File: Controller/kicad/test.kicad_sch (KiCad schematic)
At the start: 21 parts, among them J13 TEST POINTS

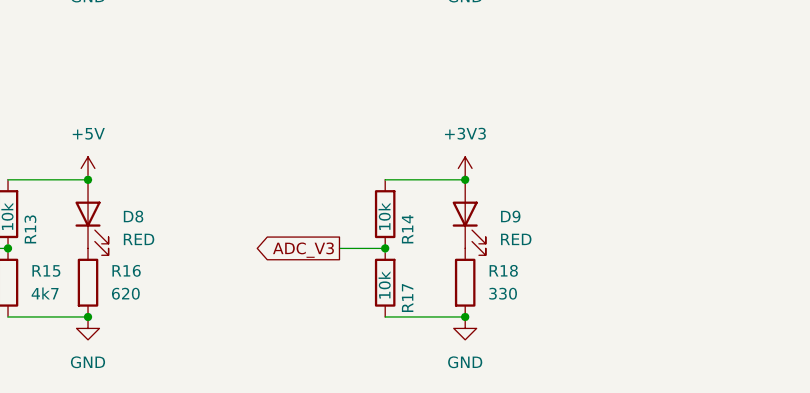
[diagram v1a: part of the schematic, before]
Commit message: Pre-production check-in
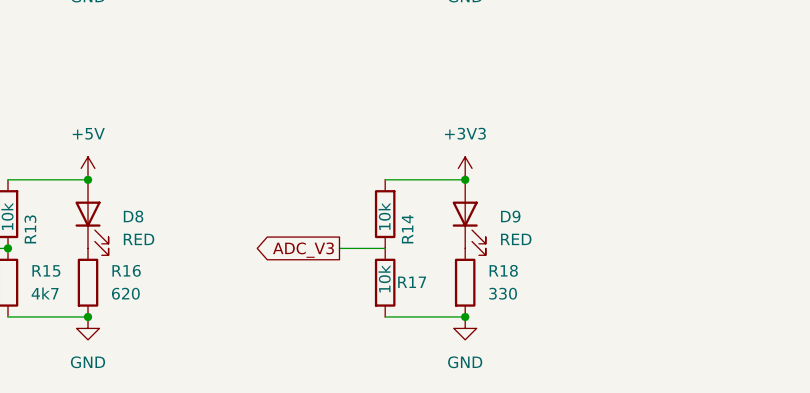
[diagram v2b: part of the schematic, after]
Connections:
- net ADC_V3: now also R17.1; no longer R17.2
- net GND: now also R17.2; no longer R17.1
- net +BATT renamed V_BATT
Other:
- moved on the sheet: R17
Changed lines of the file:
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@@
 (kicad_sch (version 20211123) (generator eeschema)
   (paper "A4")
-  (junction (at 81.28 99.06) (diameter 0) (color 0 0 0 0)
-  )
   (junction (at 39.37 58.42) (diameter 0) (color 0 0 0 0)
   )
@@
     (pin "2")
   )
-  (symbol (lib_id "Device:R") (at 81.28 102.87 180) (unit 1)
+  (symbol (lib_id "Device:R") (at 81.28 102.87 0) (unit 1)
     (in_bom yes) (on_board yes)
-    (property "Reference" "R17" (id 0) (at 83.82 102.87 90)
-      (effects (font (size 1.27 1.27)) (justify left))
-    )
-    (property "Value" "10k" (id 1) (at 81.28 101.6 90)
-      (effects (font (size 1.27 1.27)) (justify left))
-    )
-    (property "Footprint" "Resistor_SMD:R_0603_1608Metric" (id 2) (at 83.058 102.87 90)
+    (property "Reference" "R17" (id 0) (at 82.55 102.87 0)
+      (effects (font (size 1.27 1.27)) (justify left))
+    )
+    (property "Value" "10k" (id 1) (at 81.28 104.14 90)
+      (effects (font (size 1.27 1.27)) (justify left))
+    )
+    (property "Footprint" "Resistor_SMD:R_0603_1608Metric" (id 2) (at 79.502 102.87 90)
       (effects (font (size 1.27 1.27)) hide)
     )
@@
     (pin "2")
   )
-  (symbol (lib_id "Power:V_BATT") (at 90.17 50.8 0) (unit 1)
+  (symbol (lib_name "V_BATT_1") (lib_id "Power:V_BATT") (at 90.17 50.8 0) (unit 1)
     (in_bom yes) (on_board yes) (fields_autoplaced)
     (property "Reference" "#PWR038" (id 0) (at 90.17 54.61 0)
